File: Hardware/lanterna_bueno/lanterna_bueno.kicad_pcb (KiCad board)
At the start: 2 copper layers, 29.8 x 56.5 mm, 56 parts, among them J1 USB_B_Micro, Q1 BC807, Q2 2SK4075, Q3 2SK4075, Q4 2SK4075, Q5 2SK4075, U1 RT9193-33, U2 IR2101, U3 IR2101, U4 STM32F103CBTx, U5 TP4056

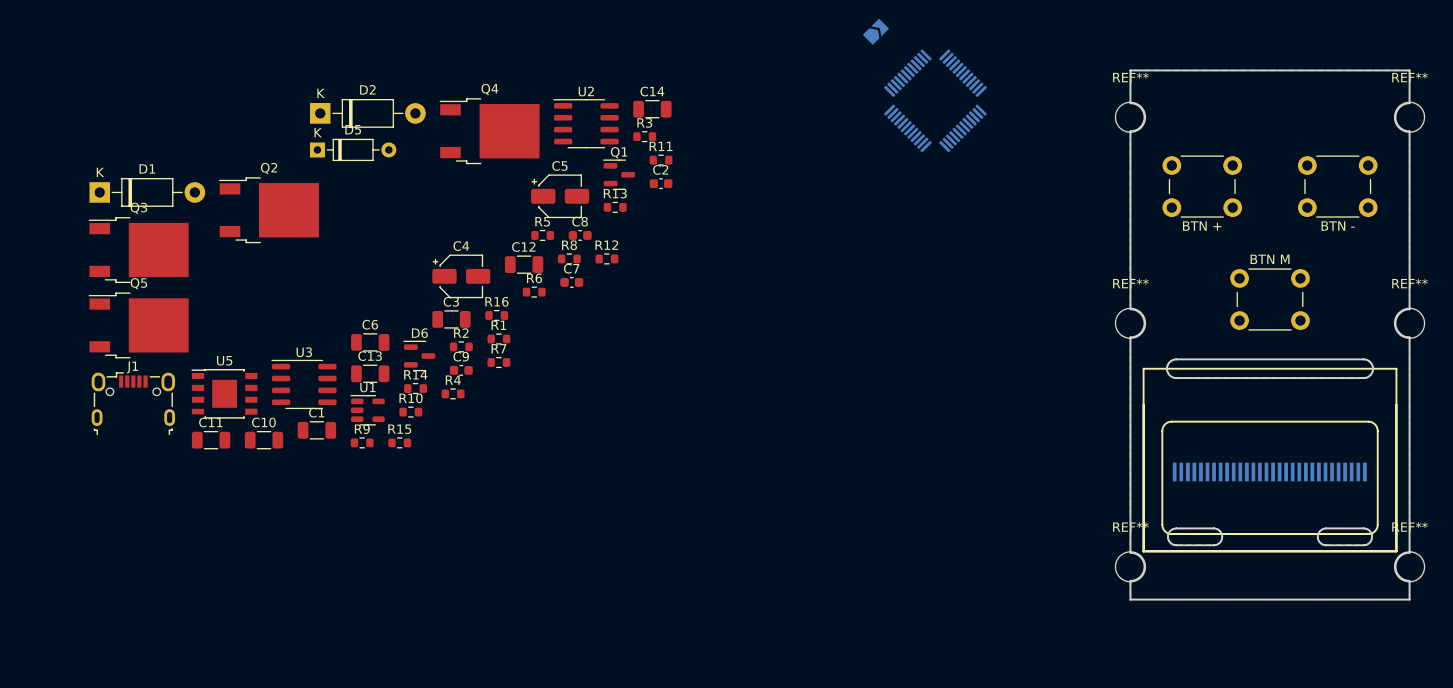
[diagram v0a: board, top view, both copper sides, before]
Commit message: building
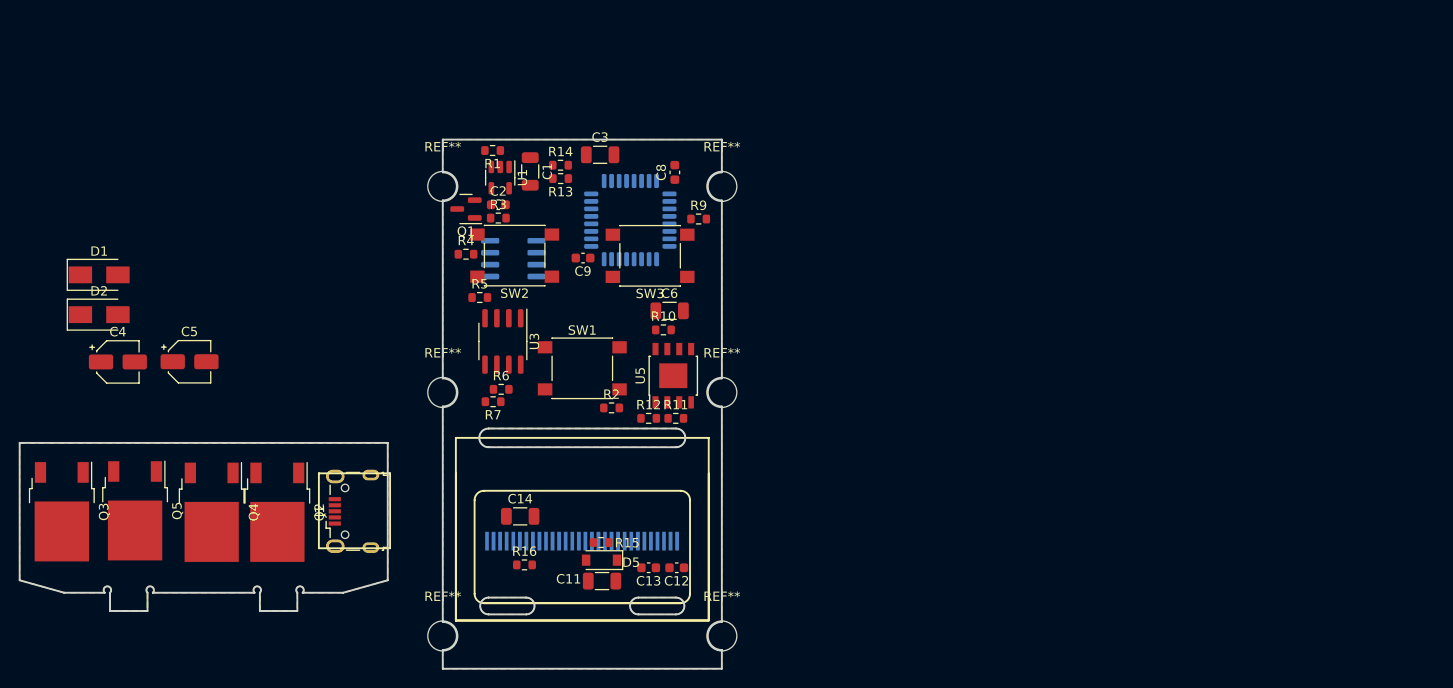
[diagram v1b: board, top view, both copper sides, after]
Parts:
- removed C10: 1uF, Capacitor_SMD:C_1206_3216Metric
- removed C7: 100nF, Capacitor_SMD:C_0603_1608Metric
- removed D6: BAT54C, Package_TO_SOT_SMD:SOT-23
- removed JP1: SolderJumper_2_Open, Jumper:SolderJumper-2_P1.3mm_Open_TrianglePad1.0x1.5mm
- removed R8: 47K, Resistor_SMD:R_0603_1608Metric
- C12, C13: footprint Capacitor_SMD:C_1206_3216Metric -> Capacitor_SMD:C_0603_1608Metric
- D1, D2: footprint Diode_THT:D_DO-41_SOD81_P10.16mm_Horizontal -> Diode_SMD:D_SMA
- D5: footprint Diode_THT:D_DO-35_SOD27_P7.62mm_Horizontal -> Diode_SMD:D_SOD-123
- SW1: renamed from BTN M; footprint Button_Switch_THT:SW_PUSH_6mm -> Button_Switch_SMD:SW_Push_1P1T_NO_6x6mm_H9.5mm
- SW2: renamed from BTN +; footprint Button_Switch_THT:SW_PUSH_6mm -> Button_Switch_SMD:SW_Push_1P1T_NO_6x6mm_H9.5mm
- SW3: renamed from BTN -; footprint Button_Switch_THT:SW_PUSH_6mm -> Button_Switch_SMD:SW_Push_1P1T_NO_6x6mm_H9.5mm
- U2: moved to B.Cu
- U4: value STM32F103CBTx -> STM32F042K6Tx; footprint Package_QFP:LQFP-48_7x7mm_P0.5mm -> Package_QFP:LQFP-32_7x7mm_P0.8mm
- moved SW3 76.8 mm to (194.8, 80.6)
- moved SW2 76.8 mm to (180.4, 80.5)
- moved REF** 73.8 mm to (202.5, 121.1)
- moved REF** 73.8 mm to (202.5, 95.1)
- moved REF** 73.8 mm to (202.5, 73.1)
- moved DS1 73.8 mm to (187.6, 111.0)
- moved REF** 73.8 mm to (172.7, 95.1)
- moved REF** 73.8 mm to (172.7, 121.1)
- moved REF** 73.8 mm to (172.7, 73.1)
- moved SW1 70.8 mm to (187.6, 92.6)
- moved D5 53.3 mm to (189.7, 113.0), turned to 180 degrees
- moved Q4 50.4 mm to (148.0, 107.9), turned to -90 degrees
- moved U5 47.9 mm to (197.3, 93.4), turned to 90 degrees
- moved C14 45.7 mm to (181.0, 108.4)
- moved C11 44.4 mm to (189.7, 115.3)
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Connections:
- U4 pad 1: VBAT -> +3V3
- U4 pad 10: BAT_MON -> unconnected-(U4-Pad10)
- U4 pad 12: unconnected-(U4-Pad12) -> PWM_LED_SUPH
- U4 pad 13: unconnected-(U4-Pad13) -> PWM_LED_SUPL
- U4 pad 14: unconnected-(U4-Pad14) -> PWM_LED_INFH
- U4 pad 15: unconnected-(U4-Pad15) -> PWM_LED_INFL
- U4 pad 16: PWM_LED_SUPH -> GND
- U4 pad 17: PWM_LED_SUPL -> +3V3
- U4 pad 18: PWM_LED_INFH -> unconnected-(U4-Pad18)
- U4 pad 19: PWM_LED_INFL -> unconnected-(U4-Pad19)
- U4 pad 2: unconnected-(U4-Pad2) -> LCD_SDA
- U4 pad 23: GND -> unconnected-(U4-Pad23)
- U4 pad 24: +3V3 -> unconnected-(U4-Pad24)
- U4 pad 25: BUT_MINUS -> unconnected-(U4-Pad25)
- U4 pad 26: BUT_PLUS -> BUT_MINUS
- U4 pad 27: BUT_MENU -> BUT_PLUS
- U4 pad 28: POWER_CMD -> BUT_MENU
- U4 pad 29: unconnected-(U4-Pad29) -> POWER_CMD
- U4 pad 3: unconnected-(U4-Pad3) -> LCD_SCL
- U4 pad 32: unconnected-(U4-Pad32) -> GND
- U4 pad 4: unconnected-(U4-Pad4) -> Net-(R9-Pad2)
- U4 pad 5: unconnected-(U4-Pad5) -> +3V3
- U4 pad 6: unconnected-(U4-Pad6) -> BAT_MON
- U4 pad 7: Net-(R9-Pad2) -> unconnected-(U4-Pad7)
- U4 pad 8: GND -> unconnected-(U4-Pad8)
- U4 pad 9: +3V3 -> unconnected-(U4-Pad9)
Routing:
- added copper zone on B.Cu, net (none)
- added copper zone on F.Cu, net (none)
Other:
- board size 29.8 x 56.5 mm -> 75 x 56.5 mm
